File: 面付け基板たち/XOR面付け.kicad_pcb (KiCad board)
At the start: 2 copper layers, 99.1 x 53.3 mm, 63 parts, among them J1 Conn_01x02, J2 Conn_01x02, J3 Conn_01x02

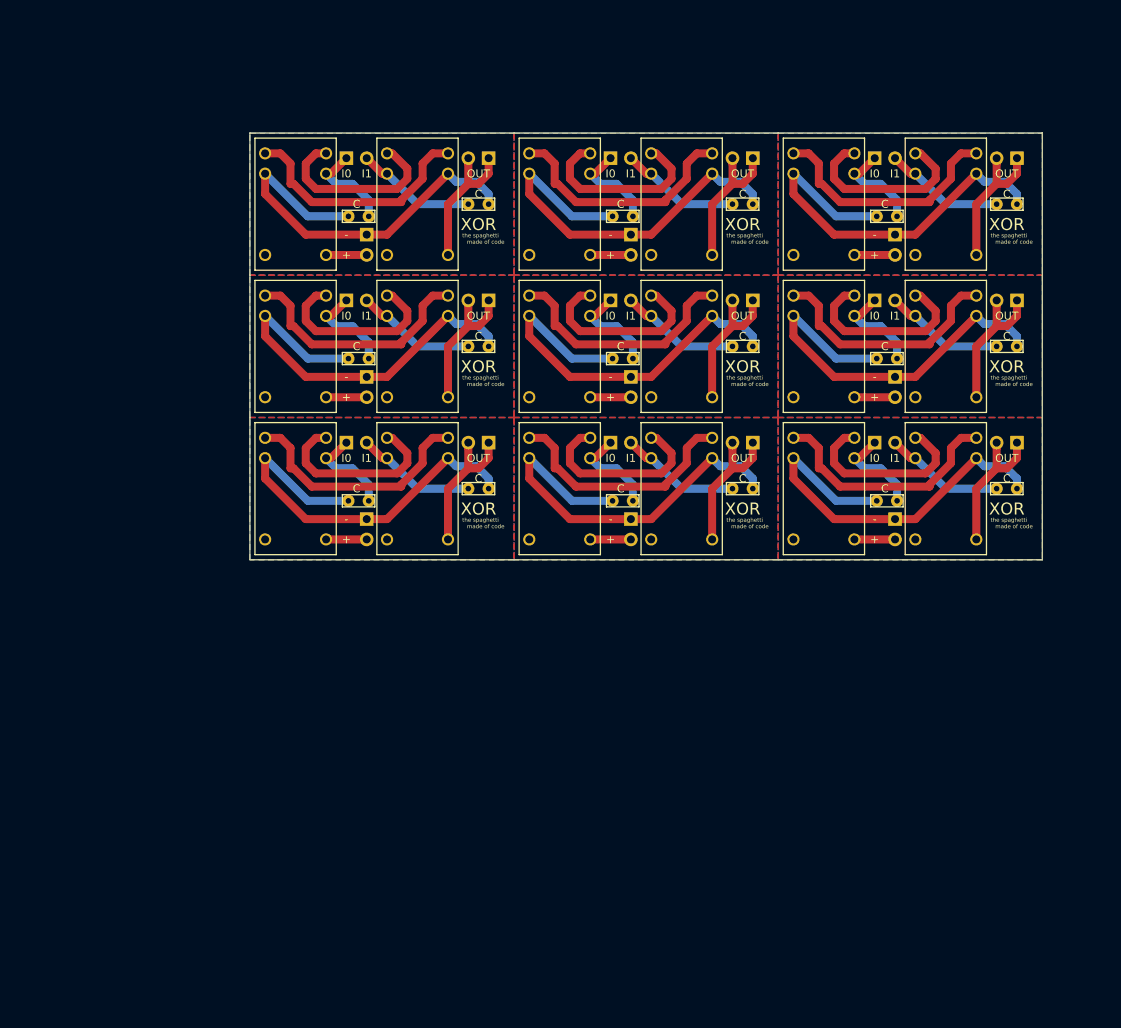
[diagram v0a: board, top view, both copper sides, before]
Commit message: Add files via upload
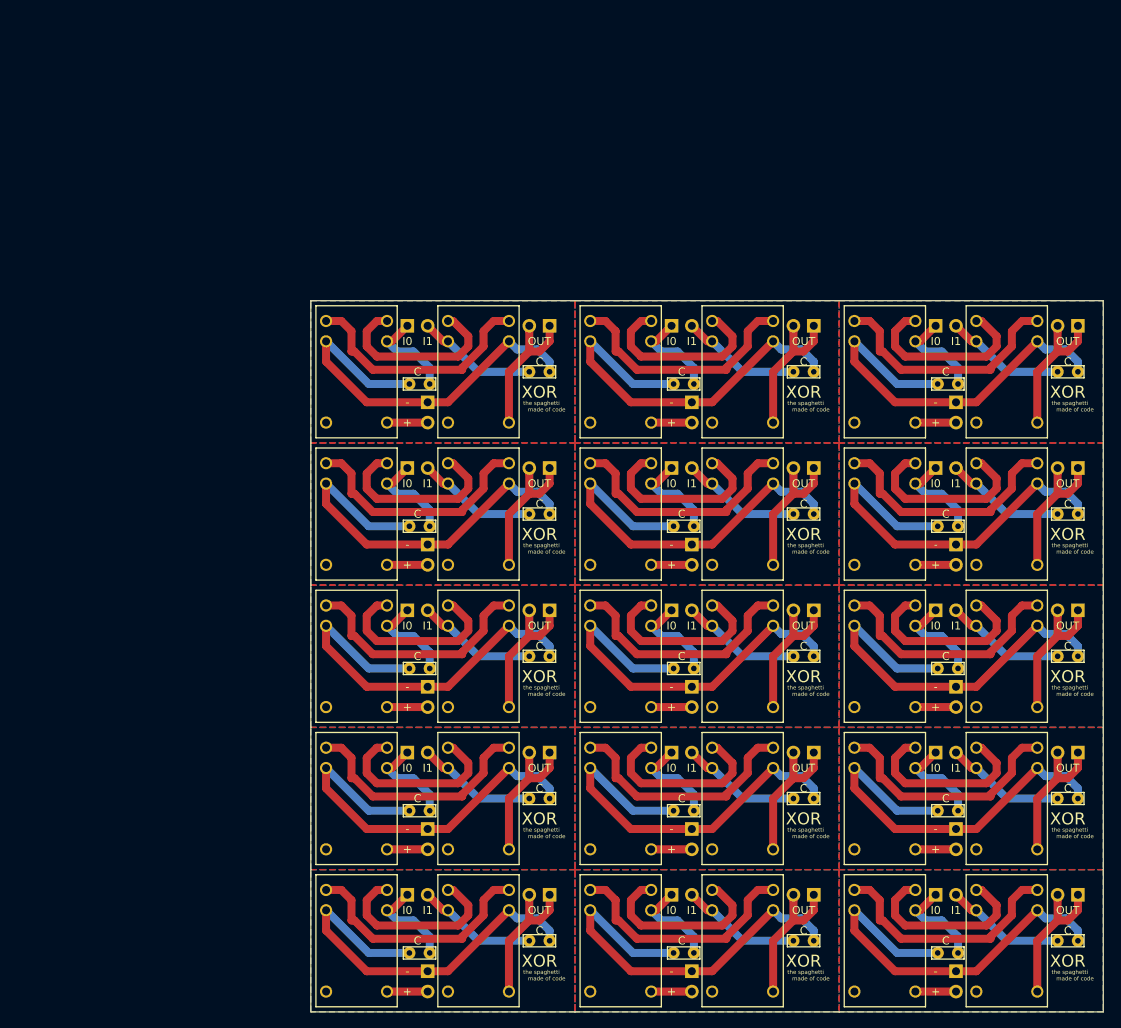
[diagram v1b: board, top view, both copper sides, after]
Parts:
- removed the C1 at (152.7, 94.2)
- removed the C1 at (119.6, 94.2)
- removed the C1 at (86.6, 94.2)
- removed the C1 at (152.7, 76.5)
- removed the C1 at (119.6, 76.5)
- removed the C1 at (86.6, 76.5)
- removed the C1 at (152.7, 58.7)
- removed the C1 at (119.6, 58.7)
- removed the C2 at (167.6, 92.7)
- removed the C2 at (134.6, 92.7)
- removed the C2 at (101.6, 92.7)
- removed the C2 at (167.6, 74.9)
- removed the C2 at (134.6, 74.9)
- removed the C2 at (101.6, 74.9)
- removed the C2 at (167.6, 57.1)
- removed the C2 at (134.6, 57.1)
- removed the J1 at (149.9, 87.0)
- removed the J1 at (116.8, 87.0)
- removed the J1 at (83.8, 87.0)
- removed the J1 at (149.9, 69.2)
- removed the J1 at (116.8, 69.2)
- removed the J1 at (83.8, 69.2)
- removed the J1 at (149.9, 51.4)
- removed the J1 at (116.8, 51.4)
- removed the J2 at (152.4, 96.5)
- removed the J2 at (119.4, 96.5)
- removed the J2 at (86.4, 96.5)
- removed the J2 at (152.4, 78.7)
- removed the J2 at (119.4, 78.7)
- removed the J2 at (86.4, 78.7)
- removed the J2 at (152.4, 61.0)
- removed the J2 at (119.4, 61.0)
- removed the J3 at (167.6, 87.0)
- removed the J3 at (134.6, 87.0)
- removed the J3 at (101.6, 87.0)
- removed the J3 at (167.6, 69.2)
- removed the J3 at (134.6, 69.2)
- removed the J3 at (101.6, 69.2)
- removed the J3 at (167.6, 51.4)
- removed the J3 at (134.6, 51.4)
- removed the SPDT1 at (144.8, 91.4)
- removed the SPDT1 at (111.8, 91.4)
- removed the SPDT1 at (78.7, 91.4)
- removed the SPDT1 at (144.8, 73.7)
- removed the SPDT1 at (111.8, 73.7)
- removed the SPDT1 at (78.7, 73.7)
- removed the SPDT1 at (144.8, 55.9)
- removed the SPDT1 at (111.8, 55.9)
- removed the SPDT2 at (160.0, 91.4)
- removed the SPDT2 at (127.0, 91.4)
- removed the SPDT2 at (94.0, 91.4)
- removed the SPDT2 at (160.0, 73.7)
- removed the SPDT2 at (127.0, 73.7)
- removed the SPDT2 at (94.0, 73.7)
- removed the SPDT2 at (160.0, 55.9)
- removed the SPDT2 at (127.0, 55.9)
- added C1: C, MiyakeFootprintLib:Condensor, F.Cu at (160.3, 150.7)
- added C1: C, MiyakeFootprintLib:Condensor, F.Cu at (160.3, 97.4)
- added C1: C, MiyakeFootprintLib:Condensor, F.Cu at (127.3, 97.4)
- added C1: C, MiyakeFootprintLib:Condensor, F.Cu at (94.2, 97.4)
- added C1: C, MiyakeFootprintLib:Condensor, F.Cu at (160.3, 79.6)
- added C1: C, MiyakeFootprintLib:Condensor, F.Cu at (127.3, 79.6)
- added C1: C, MiyakeFootprintLib:Condensor, F.Cu at (127.3, 150.7)
- added C1: C, MiyakeFootprintLib:Condensor, F.Cu at (94.2, 150.7)
- added C1: C, MiyakeFootprintLib:Condensor, F.Cu at (160.3, 133.0)
- added C1: C, MiyakeFootprintLib:Condensor, F.Cu at (127.3, 133.0)
- added C1: C, MiyakeFootprintLib:Condensor, F.Cu at (94.2, 133.0)
- added C1: C, MiyakeFootprintLib:Condensor, F.Cu at (160.3, 115.2)
- added C1: C, MiyakeFootprintLib:Condensor, F.Cu at (127.3, 115.2)
- added C1: C, MiyakeFootprintLib:Condensor, F.Cu at (94.2, 115.2)
- added C2: C, MiyakeFootprintLib:Condensor, F.Cu at (175.3, 149.2)
- added C2: C, MiyakeFootprintLib:Condensor, F.Cu at (175.3, 95.9)
- added C2: C, MiyakeFootprintLib:Condensor, F.Cu at (142.2, 95.9)
- added C2: C, MiyakeFootprintLib:Condensor, F.Cu at (109.2, 95.9)
- added C2: C, MiyakeFootprintLib:Condensor, F.Cu at (175.3, 78.1)
- added C2: C, MiyakeFootprintLib:Condensor, F.Cu at (142.2, 78.1)
- added C2: C, MiyakeFootprintLib:Condensor, F.Cu at (142.2, 149.2)
- added C2: C, MiyakeFootprintLib:Condensor, F.Cu at (109.2, 149.2)
- added C2: C, MiyakeFootprintLib:Condensor, F.Cu at (175.3, 131.4)
- added C2: C, MiyakeFootprintLib:Condensor, F.Cu at (142.2, 131.4)
- added C2: C, MiyakeFootprintLib:Condensor, F.Cu at (109.2, 131.4)
- added C2: C, MiyakeFootprintLib:Condensor, F.Cu at (175.3, 113.7)
- added C2: C, MiyakeFootprintLib:Condensor, F.Cu at (142.2, 113.7)
- added C2: C, MiyakeFootprintLib:Condensor, F.Cu at (109.2, 113.7)
- added J1: Conn_01x02, Connector_PinHeader_2.54mm:PinHeader_1x02_P2.54mm_Vertical, B.Cu at (157.5, 143.5)
- added J1: Conn_01x02, Connector_PinHeader_2.54mm:PinHeader_1x02_P2.54mm_Vertical, B.Cu at (157.5, 90.1)
- added J1: Conn_01x02, Connector_PinHeader_2.54mm:PinHeader_1x02_P2.54mm_Vertical, B.Cu at (124.5, 90.1)
- added J1: Conn_01x02, Connector_PinHeader_2.54mm:PinHeader_1x02_P2.54mm_Vertical, B.Cu at (91.4, 90.1)
- added J1: Conn_01x02, Connector_PinHeader_2.54mm:PinHeader_1x02_P2.54mm_Vertical, B.Cu at (157.5, 72.4)
- added J1: Conn_01x02, Connector_PinHeader_2.54mm:PinHeader_1x02_P2.54mm_Vertical, B.Cu at (124.5, 72.4)
- added J1: Conn_01x02, Connector_PinHeader_2.54mm:PinHeader_1x02_P2.54mm_Vertical, B.Cu at (124.5, 143.5)
- added J1: Conn_01x02, Connector_PinHeader_2.54mm:PinHeader_1x02_P2.54mm_Vertical, B.Cu at (91.4, 143.5)
- added J1: Conn_01x02, Connector_PinHeader_2.54mm:PinHeader_1x02_P2.54mm_Vertical, B.Cu at (157.5, 125.7)
- added J1: Conn_01x02, Connector_PinHeader_2.54mm:PinHeader_1x02_P2.54mm_Vertical, B.Cu at (124.5, 125.7)
- added J1: Conn_01x02, Connector_PinHeader_2.54mm:PinHeader_1x02_P2.54mm_Vertical, B.Cu at (91.4, 125.7)
- added J1: Conn_01x02, Connector_PinHeader_2.54mm:PinHeader_1x02_P2.54mm_Vertical, B.Cu at (157.5, 107.9)
- added J1: Conn_01x02, Connector_PinHeader_2.54mm:PinHeader_1x02_P2.54mm_Vertical, B.Cu at (124.5, 107.9)
- added J1: Conn_01x02, Connector_PinHeader_2.54mm:PinHeader_1x02_P2.54mm_Vertical, B.Cu at (91.4, 107.9)
- added J2: Conn_01x02, Connector_PinHeader_2.54mm:PinHeader_1x02_P2.54mm_Vertical, B.Cu at (160.0, 153.0)
- added J2: Conn_01x02, Connector_PinHeader_2.54mm:PinHeader_1x02_P2.54mm_Vertical, B.Cu at (160.0, 99.7)
- added J2: Conn_01x02, Connector_PinHeader_2.54mm:PinHeader_1x02_P2.54mm_Vertical, B.Cu at (127.0, 99.7)
- added J2: Conn_01x02, Connector_PinHeader_2.54mm:PinHeader_1x02_P2.54mm_Vertical, B.Cu at (94.0, 99.7)
- added J2: Conn_01x02, Connector_PinHeader_2.54mm:PinHeader_1x02_P2.54mm_Vertical, B.Cu at (160.0, 81.9)
- added J2: Conn_01x02, Connector_PinHeader_2.54mm:PinHeader_1x02_P2.54mm_Vertical, B.Cu at (127.0, 81.9)
- added J2: Conn_01x02, Connector_PinHeader_2.54mm:PinHeader_1x02_P2.54mm_Vertical, B.Cu at (127.0, 153.0)
- added J2: Conn_01x02, Connector_PinHeader_2.54mm:PinHeader_1x02_P2.54mm_Vertical, B.Cu at (94.0, 153.0)
- added J2: Conn_01x02, Connector_PinHeader_2.54mm:PinHeader_1x02_P2.54mm_Vertical, B.Cu at (160.0, 135.3)
- added J2: Conn_01x02, Connector_PinHeader_2.54mm:PinHeader_1x02_P2.54mm_Vertical, B.Cu at (127.0, 135.3)
- added J2: Conn_01x02, Connector_PinHeader_2.54mm:PinHeader_1x02_P2.54mm_Vertical, B.Cu at (94.0, 135.3)
- added J2: Conn_01x02, Connector_PinHeader_2.54mm:PinHeader_1x02_P2.54mm_Vertical, B.Cu at (160.0, 117.5)
- added J2: Conn_01x02, Connector_PinHeader_2.54mm:PinHeader_1x02_P2.54mm_Vertical, B.Cu at (127.0, 117.5)
- added J2: Conn_01x02, Connector_PinHeader_2.54mm:PinHeader_1x02_P2.54mm_Vertical, B.Cu at (94.0, 117.5)
- added J3: Conn_01x02, Connector_PinHeader_2.54mm:PinHeader_1x02_P2.54mm_Vertical, B.Cu at (175.3, 143.5)
- added J3: Conn_01x02, Connector_PinHeader_2.54mm:PinHeader_1x02_P2.54mm_Vertical, B.Cu at (175.3, 90.1)
- added J3: Conn_01x02, Connector_PinHeader_2.54mm:PinHeader_1x02_P2.54mm_Vertical, B.Cu at (142.2, 90.1)
- added J3: Conn_01x02, Connector_PinHeader_2.54mm:PinHeader_1x02_P2.54mm_Vertical, B.Cu at (109.2, 90.1)
- added J3: Conn_01x02, Connector_PinHeader_2.54mm:PinHeader_1x02_P2.54mm_Vertical, B.Cu at (175.3, 72.4)
- added J3: Conn_01x02, Connector_PinHeader_2.54mm:PinHeader_1x02_P2.54mm_Vertical, B.Cu at (142.2, 72.4)
- added J3: Conn_01x02, Connector_PinHeader_2.54mm:PinHeader_1x02_P2.54mm_Vertical, B.Cu at (142.2, 143.5)
- added J3: Conn_01x02, Connector_PinHeader_2.54mm:PinHeader_1x02_P2.54mm_Vertical, B.Cu at (109.2, 143.5)
- added J3: Conn_01x02, Connector_PinHeader_2.54mm:PinHeader_1x02_P2.54mm_Vertical, B.Cu at (175.3, 125.7)
- added J3: Conn_01x02, Connector_PinHeader_2.54mm:PinHeader_1x02_P2.54mm_Vertical, B.Cu at (142.2, 125.7)
- added J3: Conn_01x02, Connector_PinHeader_2.54mm:PinHeader_1x02_P2.54mm_Vertical, B.Cu at (109.2, 125.7)
- added J3: Conn_01x02, Connector_PinHeader_2.54mm:PinHeader_1x02_P2.54mm_Vertical, B.Cu at (175.3, 107.9)
- added J3: Conn_01x02, Connector_PinHeader_2.54mm:PinHeader_1x02_P2.54mm_Vertical, B.Cu at (142.2, 107.9)
- added J3: Conn_01x02, Connector_PinHeader_2.54mm:PinHeader_1x02_P2.54mm_Vertical, B.Cu at (109.2, 107.9)
- added SPDT1: 946H-1C-24D, MiyakeFootprintLib:946H-1C-24D, F.Cu at (152.4, 148.0)
- added SPDT1: 946H-1C-24D, MiyakeFootprintLib:946H-1C-24D, F.Cu at (152.4, 94.6)
- added SPDT1: 946H-1C-24D, MiyakeFootprintLib:946H-1C-24D, F.Cu at (119.4, 94.6)
- added SPDT1: 946H-1C-24D, MiyakeFootprintLib:946H-1C-24D, F.Cu at (86.4, 94.6)
- added SPDT1: 946H-1C-24D, MiyakeFootprintLib:946H-1C-24D, F.Cu at (152.4, 76.8)
- added SPDT1: 946H-1C-24D, MiyakeFootprintLib:946H-1C-24D, F.Cu at (119.4, 76.8)
- added SPDT1: 946H-1C-24D, MiyakeFootprintLib:946H-1C-24D, F.Cu at (119.4, 148.0)
- added SPDT1: 946H-1C-24D, MiyakeFootprintLib:946H-1C-24D, F.Cu at (86.4, 148.0)
- added SPDT1: 946H-1C-24D, MiyakeFootprintLib:946H-1C-24D, F.Cu at (152.4, 130.2)
- added SPDT1: 946H-1C-24D, MiyakeFootprintLib:946H-1C-24D, F.Cu at (119.4, 130.2)
- added SPDT1: 946H-1C-24D, MiyakeFootprintLib:946H-1C-24D, F.Cu at (86.4, 130.2)
- added SPDT1: 946H-1C-24D, MiyakeFootprintLib:946H-1C-24D, F.Cu at (152.4, 112.4)
- added SPDT1: 946H-1C-24D, MiyakeFootprintLib:946H-1C-24D, F.Cu at (119.4, 112.4)
- added SPDT1: 946H-1C-24D, MiyakeFootprintLib:946H-1C-24D, F.Cu at (86.4, 112.4)
- added SPDT2: 946H-1C-24D, MiyakeFootprintLib:946H-1C-24D, F.Cu at (167.6, 148.0)
- added SPDT2: 946H-1C-24D, MiyakeFootprintLib:946H-1C-24D, F.Cu at (167.6, 94.6)
- added SPDT2: 946H-1C-24D, MiyakeFootprintLib:946H-1C-24D, F.Cu at (134.6, 94.6)
- added SPDT2: 946H-1C-24D, MiyakeFootprintLib:946H-1C-24D, F.Cu at (101.6, 94.6)
- added SPDT2: 946H-1C-24D, MiyakeFootprintLib:946H-1C-24D, F.Cu at (167.6, 76.8)
- added SPDT2: 946H-1C-24D, MiyakeFootprintLib:946H-1C-24D, F.Cu at (134.6, 76.8)
- added SPDT2: 946H-1C-24D, MiyakeFootprintLib:946H-1C-24D, F.Cu at (134.6, 148.0)
- added SPDT2: 946H-1C-24D, MiyakeFootprintLib:946H-1C-24D, F.Cu at (101.6, 148.0)
- added SPDT2: 946H-1C-24D, MiyakeFootprintLib:946H-1C-24D, F.Cu at (167.6, 130.2)
- added SPDT2: 946H-1C-24D, MiyakeFootprintLib:946H-1C-24D, F.Cu at (134.6, 130.2)
- added SPDT2: 946H-1C-24D, MiyakeFootprintLib:946H-1C-24D, F.Cu at (101.6, 130.2)
- added SPDT2: 946H-1C-24D, MiyakeFootprintLib:946H-1C-24D, F.Cu at (167.6, 112.4)
- added SPDT2: 946H-1C-24D, MiyakeFootprintLib:946H-1C-24D, F.Cu at (134.6, 112.4)
- added SPDT2: 946H-1C-24D, MiyakeFootprintLib:946H-1C-24D, F.Cu at (101.6, 112.4)
- moved C2 22.3 mm to (109.2, 78.1)
- moved J1 22.3 mm to (91.4, 72.4)
- moved J2 22.3 mm to (94.0, 81.9)
- moved J3 22.3 mm to (109.2, 72.4)
- moved C1 22.3 mm to (94.2, 79.6)
- moved SPDT1 22.3 mm to (86.4, 76.8)
- moved SPDT2 22.3 mm to (101.6, 76.8)
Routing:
- net GND: track 456.2 -> 760.3 mm
- net Net-(SPDT1-Pad1): track 276.0 -> 459.9 mm
- net Net-(SPDT1-Pad2): track 209.9 -> 349.8 mm
- net Net-(J3-Pad1): track 163.4 -> 272.4 mm
- net Net-(C2-Pad2): track 135.7 -> 226.2 mm
- net Net-(C1-Pad1): track 108.7 -> 181.2 mm
- net +24V: track 45.7 -> 76.2 mm
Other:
- board size 99.1 x 53.3 mm -> 99.1 x 88.9 mm

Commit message: Add files via upload
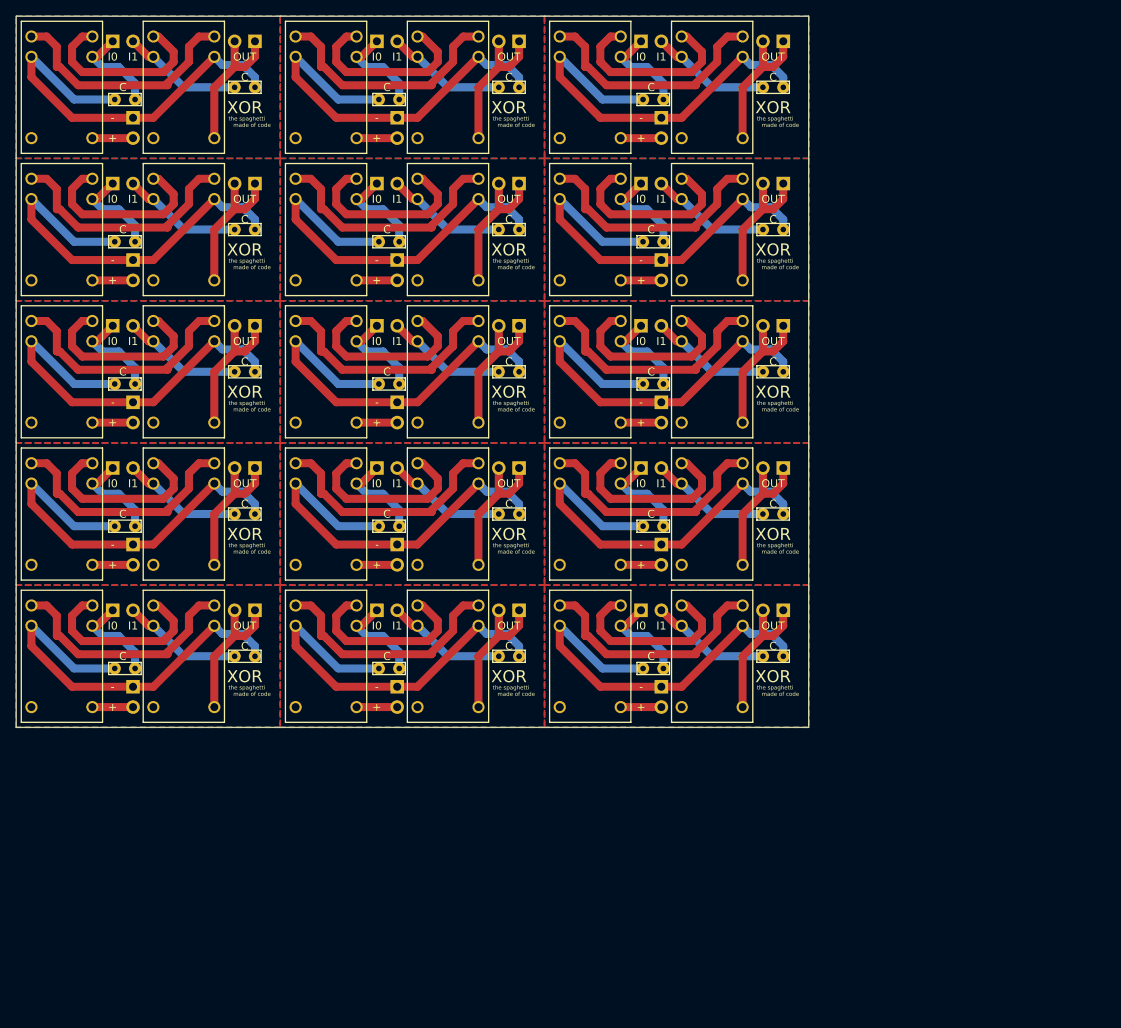
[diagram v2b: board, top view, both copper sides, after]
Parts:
- removed the C1 at (160.3, 150.7)
- removed the C1 at (160.3, 97.4)
- removed the C1 at (127.3, 97.4)
- removed the C1 at (94.2, 97.4)
- removed the C1 at (160.3, 79.6)
- removed the C1 at (127.3, 79.6)
- removed the C1 at (127.3, 150.7)
- removed the C1 at (94.2, 150.7)
- removed the C1 at (160.3, 133.0)
- removed the C1 at (127.3, 133.0)
- removed the C1 at (94.2, 133.0)
- removed the C1 at (160.3, 115.2)
- removed the C1 at (127.3, 115.2)
- removed the C1 at (94.2, 115.2)
- removed the C2 at (175.3, 149.2)
- removed the C2 at (175.3, 95.9)
- removed the C2 at (142.2, 95.9)
- removed the C2 at (109.2, 95.9)
- removed the C2 at (175.3, 78.1)
- removed the C2 at (142.2, 78.1)
- removed the C2 at (142.2, 149.2)
- removed the C2 at (109.2, 149.2)
- removed the C2 at (175.3, 131.4)
- removed the C2 at (142.2, 131.4)
- removed the C2 at (109.2, 131.4)
- removed the C2 at (175.3, 113.7)
- removed the C2 at (142.2, 113.7)
- removed the C2 at (109.2, 113.7)
- removed the J1 at (157.5, 143.5)
- removed the J1 at (157.5, 90.1)
- removed the J1 at (124.5, 90.1)
- removed the J1 at (91.4, 90.1)
- removed the J1 at (157.5, 72.4)
- removed the J1 at (124.5, 72.4)
- removed the J1 at (124.5, 143.5)
- removed the J1 at (91.4, 143.5)
- removed the J1 at (157.5, 125.7)
- removed the J1 at (124.5, 125.7)
- removed the J1 at (91.4, 125.7)
- removed the J1 at (157.5, 107.9)
- removed the J1 at (124.5, 107.9)
- removed the J1 at (91.4, 107.9)
- removed the J2 at (160.0, 153.0)
- removed the J2 at (160.0, 99.7)
- removed the J2 at (127.0, 99.7)
- removed the J2 at (94.0, 99.7)
- removed the J2 at (160.0, 81.9)
- removed the J2 at (127.0, 81.9)
- removed the J2 at (127.0, 153.0)
- removed the J2 at (94.0, 153.0)
- removed the J2 at (160.0, 135.3)
- removed the J2 at (127.0, 135.3)
- removed the J2 at (94.0, 135.3)
- removed the J2 at (160.0, 117.5)
- removed the J2 at (127.0, 117.5)
- removed the J2 at (94.0, 117.5)
- removed the J3 at (175.3, 143.5)
- removed the J3 at (175.3, 90.1)
- removed the J3 at (142.2, 90.1)
- removed the J3 at (109.2, 90.1)
- removed the J3 at (175.3, 72.4)
- removed the J3 at (142.2, 72.4)
- removed the J3 at (142.2, 143.5)
- removed the J3 at (109.2, 143.5)
- removed the J3 at (175.3, 125.7)
- removed the J3 at (142.2, 125.7)
- removed the J3 at (109.2, 125.7)
- removed the J3 at (175.3, 107.9)
- removed the J3 at (142.2, 107.9)
- removed the J3 at (109.2, 107.9)
- removed the SPDT1 at (152.4, 148.0)
- removed the SPDT1 at (152.4, 94.6)
- removed the SPDT1 at (119.4, 94.6)
- removed the SPDT1 at (86.4, 94.6)
- removed the SPDT1 at (152.4, 76.8)
- removed the SPDT1 at (119.4, 76.8)
- removed the SPDT1 at (119.4, 148.0)
- removed the SPDT1 at (86.4, 148.0)
- removed the SPDT1 at (152.4, 130.2)
- removed the SPDT1 at (119.4, 130.2)
- removed the SPDT1 at (86.4, 130.2)
- removed the SPDT1 at (152.4, 112.4)
- removed the SPDT1 at (119.4, 112.4)
- removed the SPDT1 at (86.4, 112.4)
- removed the SPDT2 at (167.6, 148.0)
- removed the SPDT2 at (167.6, 94.6)
- removed the SPDT2 at (134.6, 94.6)
- removed the SPDT2 at (101.6, 94.6)
- removed the SPDT2 at (167.6, 76.8)
- removed the SPDT2 at (134.6, 76.8)
- removed the SPDT2 at (134.6, 148.0)
- removed the SPDT2 at (101.6, 148.0)
- removed the SPDT2 at (167.6, 130.2)
- removed the SPDT2 at (134.6, 130.2)
- removed the SPDT2 at (101.6, 130.2)
- removed the SPDT2 at (167.6, 112.4)
- removed the SPDT2 at (134.6, 112.4)
- removed the SPDT2 at (101.6, 112.4)
- added C1: C, MiyakeFootprintLib:Condensor, F.Cu at (123.4, 115.2)
- added C1: C, MiyakeFootprintLib:Condensor, F.Cu at (123.4, 61.8)
- added C1: C, MiyakeFootprintLib:Condensor, F.Cu at (90.4, 61.8)
- added C1: C, MiyakeFootprintLib:Condensor, F.Cu at (57.4, 61.8)
- added C1: C, MiyakeFootprintLib:Condensor, F.Cu at (123.4, 44.1)
- added C1: C, MiyakeFootprintLib:Condensor, F.Cu at (90.4, 44.1)
- added C1: C, MiyakeFootprintLib:Condensor, F.Cu at (90.4, 115.2)
- added C1: C, MiyakeFootprintLib:Condensor, F.Cu at (57.4, 115.2)
- added C1: C, MiyakeFootprintLib:Condensor, F.Cu at (123.4, 97.4)
- added C1: C, MiyakeFootprintLib:Condensor, F.Cu at (90.4, 97.4)
- added C1: C, MiyakeFootprintLib:Condensor, F.Cu at (57.4, 97.4)
- added C1: C, MiyakeFootprintLib:Condensor, F.Cu at (123.4, 79.6)
- added C1: C, MiyakeFootprintLib:Condensor, F.Cu at (90.4, 79.6)
- added C1: C, MiyakeFootprintLib:Condensor, F.Cu at (57.4, 79.6)
- added C2: C, MiyakeFootprintLib:Condensor, F.Cu at (138.4, 113.7)
- added C2: C, MiyakeFootprintLib:Condensor, F.Cu at (138.4, 60.3)
- added C2: C, MiyakeFootprintLib:Condensor, F.Cu at (105.4, 60.3)
- added C2: C, MiyakeFootprintLib:Condensor, F.Cu at (72.4, 60.3)
- added C2: C, MiyakeFootprintLib:Condensor, F.Cu at (138.4, 42.5)
- added C2: C, MiyakeFootprintLib:Condensor, F.Cu at (105.4, 42.5)
- added C2: C, MiyakeFootprintLib:Condensor, F.Cu at (105.4, 113.7)
- added C2: C, MiyakeFootprintLib:Condensor, F.Cu at (72.4, 113.7)
- added C2: C, MiyakeFootprintLib:Condensor, F.Cu at (138.4, 95.9)
- added C2: C, MiyakeFootprintLib:Condensor, F.Cu at (105.4, 95.9)
- added C2: C, MiyakeFootprintLib:Condensor, F.Cu at (72.4, 95.9)
- added C2: C, MiyakeFootprintLib:Condensor, F.Cu at (138.4, 78.1)
- added C2: C, MiyakeFootprintLib:Condensor, F.Cu at (105.4, 78.1)
- added C2: C, MiyakeFootprintLib:Condensor, F.Cu at (72.4, 78.1)
- added J1: Conn_01x02, Connector_PinHeader_2.54mm:PinHeader_1x02_P2.54mm_Vertical, B.Cu at (120.7, 107.9)
- added J1: Conn_01x02, Connector_PinHeader_2.54mm:PinHeader_1x02_P2.54mm_Vertical, B.Cu at (120.7, 54.6)
- added J1: Conn_01x02, Connector_PinHeader_2.54mm:PinHeader_1x02_P2.54mm_Vertical, B.Cu at (87.6, 54.6)
- added J1: Conn_01x02, Connector_PinHeader_2.54mm:PinHeader_1x02_P2.54mm_Vertical, B.Cu at (54.6, 54.6)
- added J1: Conn_01x02, Connector_PinHeader_2.54mm:PinHeader_1x02_P2.54mm_Vertical, B.Cu at (120.7, 36.8)
- added J1: Conn_01x02, Connector_PinHeader_2.54mm:PinHeader_1x02_P2.54mm_Vertical, B.Cu at (87.6, 36.8)
- added J1: Conn_01x02, Connector_PinHeader_2.54mm:PinHeader_1x02_P2.54mm_Vertical, B.Cu at (87.6, 107.9)
- added J1: Conn_01x02, Connector_PinHeader_2.54mm:PinHeader_1x02_P2.54mm_Vertical, B.Cu at (54.6, 107.9)
- added J1: Conn_01x02, Connector_PinHeader_2.54mm:PinHeader_1x02_P2.54mm_Vertical, B.Cu at (120.7, 90.1)
- added J1: Conn_01x02, Connector_PinHeader_2.54mm:PinHeader_1x02_P2.54mm_Vertical, B.Cu at (87.6, 90.1)
- added J1: Conn_01x02, Connector_PinHeader_2.54mm:PinHeader_1x02_P2.54mm_Vertical, B.Cu at (54.6, 90.1)
- added J1: Conn_01x02, Connector_PinHeader_2.54mm:PinHeader_1x02_P2.54mm_Vertical, B.Cu at (120.7, 72.4)
- added J1: Conn_01x02, Connector_PinHeader_2.54mm:PinHeader_1x02_P2.54mm_Vertical, B.Cu at (87.6, 72.4)
- added J1: Conn_01x02, Connector_PinHeader_2.54mm:PinHeader_1x02_P2.54mm_Vertical, B.Cu at (54.6, 72.4)
- added J2: Conn_01x02, Connector_PinHeader_2.54mm:PinHeader_1x02_P2.54mm_Vertical, B.Cu at (123.2, 117.5)
- added J2: Conn_01x02, Connector_PinHeader_2.54mm:PinHeader_1x02_P2.54mm_Vertical, B.Cu at (123.2, 64.1)
- added J2: Conn_01x02, Connector_PinHeader_2.54mm:PinHeader_1x02_P2.54mm_Vertical, B.Cu at (90.2, 64.1)
- added J2: Conn_01x02, Connector_PinHeader_2.54mm:PinHeader_1x02_P2.54mm_Vertical, B.Cu at (57.1, 64.1)
- added J2: Conn_01x02, Connector_PinHeader_2.54mm:PinHeader_1x02_P2.54mm_Vertical, B.Cu at (123.2, 46.4)
- added J2: Conn_01x02, Connector_PinHeader_2.54mm:PinHeader_1x02_P2.54mm_Vertical, B.Cu at (90.2, 46.4)
- added J2: Conn_01x02, Connector_PinHeader_2.54mm:PinHeader_1x02_P2.54mm_Vertical, B.Cu at (90.2, 117.5)
- added J2: Conn_01x02, Connector_PinHeader_2.54mm:PinHeader_1x02_P2.54mm_Vertical, B.Cu at (57.1, 117.5)
- added J2: Conn_01x02, Connector_PinHeader_2.54mm:PinHeader_1x02_P2.54mm_Vertical, B.Cu at (123.2, 99.7)
- added J2: Conn_01x02, Connector_PinHeader_2.54mm:PinHeader_1x02_P2.54mm_Vertical, B.Cu at (90.2, 99.7)
- added J2: Conn_01x02, Connector_PinHeader_2.54mm:PinHeader_1x02_P2.54mm_Vertical, B.Cu at (57.1, 99.7)
- added J2: Conn_01x02, Connector_PinHeader_2.54mm:PinHeader_1x02_P2.54mm_Vertical, B.Cu at (123.2, 81.9)
- added J2: Conn_01x02, Connector_PinHeader_2.54mm:PinHeader_1x02_P2.54mm_Vertical, B.Cu at (90.2, 81.9)
- added J2: Conn_01x02, Connector_PinHeader_2.54mm:PinHeader_1x02_P2.54mm_Vertical, B.Cu at (57.1, 81.9)
- added J3: Conn_01x02, Connector_PinHeader_2.54mm:PinHeader_1x02_P2.54mm_Vertical, B.Cu at (138.4, 107.9)
- added J3: Conn_01x02, Connector_PinHeader_2.54mm:PinHeader_1x02_P2.54mm_Vertical, B.Cu at (138.4, 54.6)
- added J3: Conn_01x02, Connector_PinHeader_2.54mm:PinHeader_1x02_P2.54mm_Vertical, B.Cu at (105.4, 54.6)
- added J3: Conn_01x02, Connector_PinHeader_2.54mm:PinHeader_1x02_P2.54mm_Vertical, B.Cu at (72.4, 54.6)
- added J3: Conn_01x02, Connector_PinHeader_2.54mm:PinHeader_1x02_P2.54mm_Vertical, B.Cu at (138.4, 36.8)
- added J3: Conn_01x02, Connector_PinHeader_2.54mm:PinHeader_1x02_P2.54mm_Vertical, B.Cu at (105.4, 36.8)
- added J3: Conn_01x02, Connector_PinHeader_2.54mm:PinHeader_1x02_P2.54mm_Vertical, B.Cu at (105.4, 107.9)
- added J3: Conn_01x02, Connector_PinHeader_2.54mm:PinHeader_1x02_P2.54mm_Vertical, B.Cu at (72.4, 107.9)
- added J3: Conn_01x02, Connector_PinHeader_2.54mm:PinHeader_1x02_P2.54mm_Vertical, B.Cu at (138.4, 90.1)
- added J3: Conn_01x02, Connector_PinHeader_2.54mm:PinHeader_1x02_P2.54mm_Vertical, B.Cu at (105.4, 90.1)
- added J3: Conn_01x02, Connector_PinHeader_2.54mm:PinHeader_1x02_P2.54mm_Vertical, B.Cu at (72.4, 90.1)
- added J3: Conn_01x02, Connector_PinHeader_2.54mm:PinHeader_1x02_P2.54mm_Vertical, B.Cu at (138.4, 72.4)
- added J3: Conn_01x02, Connector_PinHeader_2.54mm:PinHeader_1x02_P2.54mm_Vertical, B.Cu at (105.4, 72.4)
- added J3: Conn_01x02, Connector_PinHeader_2.54mm:PinHeader_1x02_P2.54mm_Vertical, B.Cu at (72.4, 72.4)
- added SPDT1: 946H-1C-24D, MiyakeFootprintLib:946H-1C-24D, F.Cu at (115.6, 112.4)
- added SPDT1: 946H-1C-24D, MiyakeFootprintLib:946H-1C-24D, F.Cu at (115.6, 59.1)
- added SPDT1: 946H-1C-24D, MiyakeFootprintLib:946H-1C-24D, F.Cu at (82.5, 59.1)
- added SPDT1: 946H-1C-24D, MiyakeFootprintLib:946H-1C-24D, F.Cu at (49.5, 59.1)
- added SPDT1: 946H-1C-24D, MiyakeFootprintLib:946H-1C-24D, F.Cu at (115.6, 41.3)
- added SPDT1: 946H-1C-24D, MiyakeFootprintLib:946H-1C-24D, F.Cu at (82.5, 41.3)
- added SPDT1: 946H-1C-24D, MiyakeFootprintLib:946H-1C-24D, F.Cu at (82.5, 112.4)
- added SPDT1: 946H-1C-24D, MiyakeFootprintLib:946H-1C-24D, F.Cu at (49.5, 112.4)
- added SPDT1: 946H-1C-24D, MiyakeFootprintLib:946H-1C-24D, F.Cu at (115.6, 94.6)
- added SPDT1: 946H-1C-24D, MiyakeFootprintLib:946H-1C-24D, F.Cu at (82.5, 94.6)
- added SPDT1: 946H-1C-24D, MiyakeFootprintLib:946H-1C-24D, F.Cu at (49.5, 94.6)
- added SPDT1: 946H-1C-24D, MiyakeFootprintLib:946H-1C-24D, F.Cu at (115.6, 76.8)
- added SPDT1: 946H-1C-24D, MiyakeFootprintLib:946H-1C-24D, F.Cu at (82.5, 76.8)
- added SPDT1: 946H-1C-24D, MiyakeFootprintLib:946H-1C-24D, F.Cu at (49.5, 76.8)
- added SPDT2: 946H-1C-24D, MiyakeFootprintLib:946H-1C-24D, F.Cu at (130.8, 112.4)
- added SPDT2: 946H-1C-24D, MiyakeFootprintLib:946H-1C-24D, F.Cu at (130.8, 59.1)
- added SPDT2: 946H-1C-24D, MiyakeFootprintLib:946H-1C-24D, F.Cu at (97.8, 59.1)
- added SPDT2: 946H-1C-24D, MiyakeFootprintLib:946H-1C-24D, F.Cu at (64.8, 59.1)
- added SPDT2: 946H-1C-24D, MiyakeFootprintLib:946H-1C-24D, F.Cu at (130.8, 41.3)
- added SPDT2: 946H-1C-24D, MiyakeFootprintLib:946H-1C-24D, F.Cu at (97.8, 41.3)
- added SPDT2: 946H-1C-24D, MiyakeFootprintLib:946H-1C-24D, F.Cu at (97.8, 112.4)
- added SPDT2: 946H-1C-24D, MiyakeFootprintLib:946H-1C-24D, F.Cu at (64.8, 112.4)
- added SPDT2: 946H-1C-24D, MiyakeFootprintLib:946H-1C-24D, F.Cu at (130.8, 94.6)
- added SPDT2: 946H-1C-24D, MiyakeFootprintLib:946H-1C-24D, F.Cu at (97.8, 94.6)
- added SPDT2: 946H-1C-24D, MiyakeFootprintLib:946H-1C-24D, F.Cu at (64.8, 94.6)
- added SPDT2: 946H-1C-24D, MiyakeFootprintLib:946H-1C-24D, F.Cu at (130.8, 76.8)
- added SPDT2: 946H-1C-24D, MiyakeFootprintLib:946H-1C-24D, F.Cu at (97.8, 76.8)
- added SPDT2: 946H-1C-24D, MiyakeFootprintLib:946H-1C-24D, F.Cu at (64.8, 76.8)
- moved J2 51.2 mm to (57.1, 46.4)
- moved C2 51.2 mm to (72.4, 42.5)
- moved J1 51.2 mm to (54.6, 36.8)
- moved J3 51.2 mm to (72.4, 36.8)
- moved C1 51.2 mm to (57.4, 44.1)
- moved SPDT1 51.2 mm to (49.5, 41.3)
- moved SPDT2 51.2 mm to (64.8, 41.3)
